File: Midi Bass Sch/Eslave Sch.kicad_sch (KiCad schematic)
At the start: 12 parts, among them J3 E SLAVE ISCP, SW3 E-slave Reset, U2 PIC16F1789

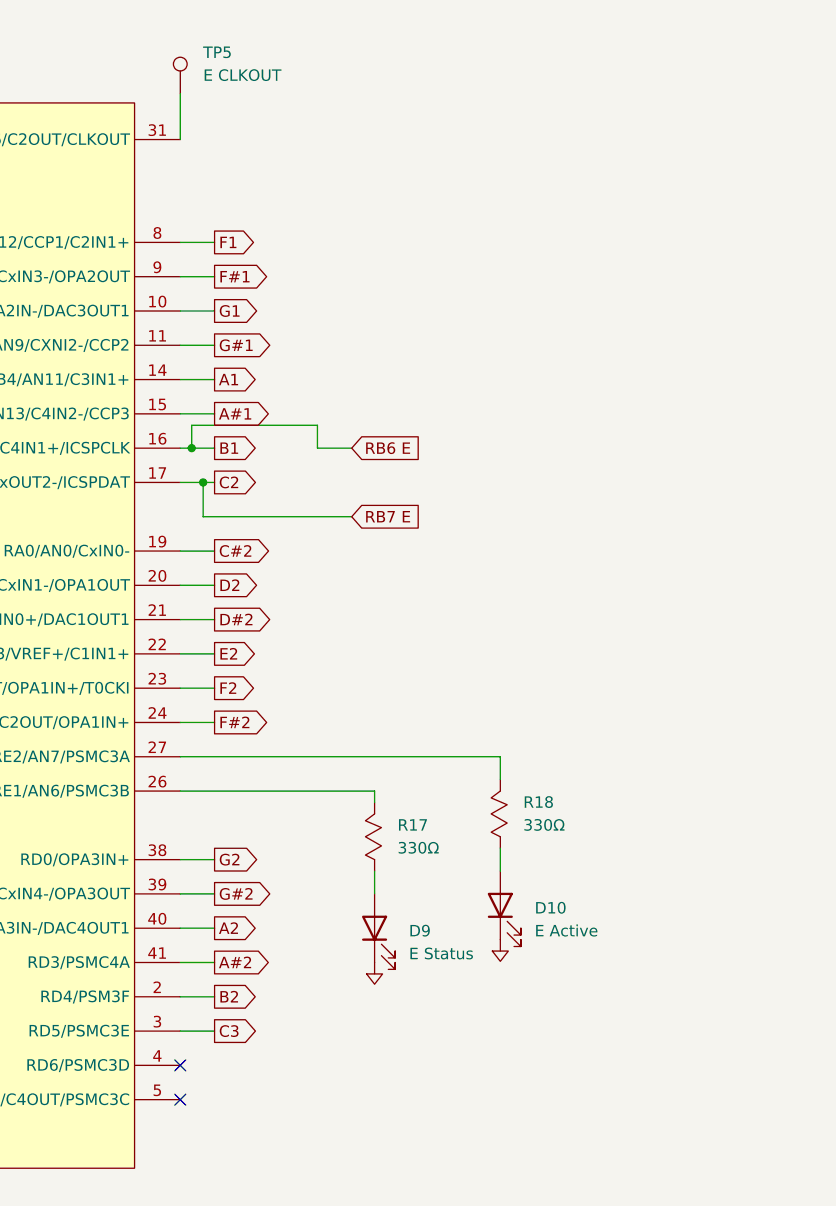
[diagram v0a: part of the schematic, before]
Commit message: finished troubleshooting section
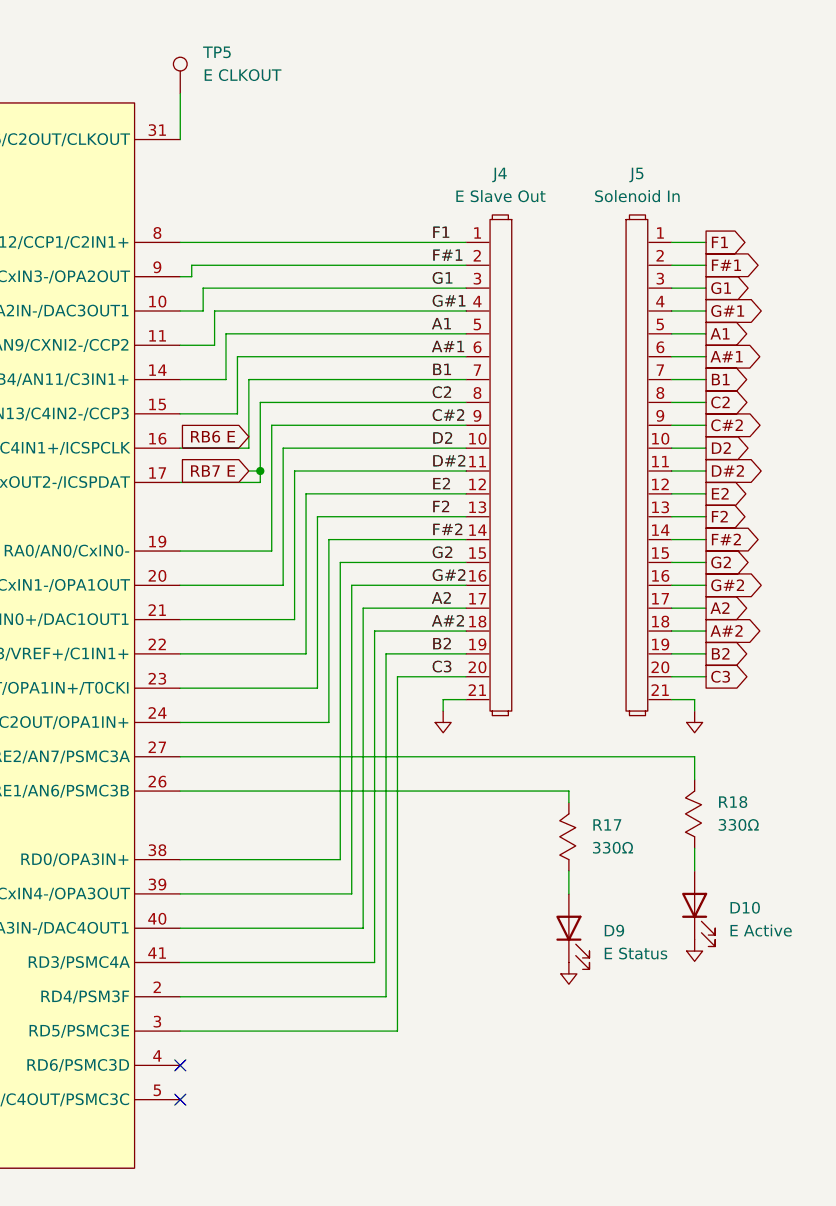
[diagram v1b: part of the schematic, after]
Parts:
- added J4: E Slave Out, symbol Owen's Symbols:Header_1x21
- added J5: Solenoid In, symbol Owen's Symbols:Header_1x21
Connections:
- net A#1: now also J4.6, J5.6
- net A#2: now also J4.18, J5.18
- net A1: now also J4.5, J5.5
- net A2: now also J4.17, J5.17
- net B1: now also J4.7, J5.7
- net B2: now also J4.19, J5.19
- net C#2: now also J4.9, J5.9
- net C2: now also J4.8, J5.8
- net C3: now also J4.20, J5.20
- net D#2: now also J4.11, J5.11
- net D2: now also J4.10, J5.10
- net E2: now also J4.12, J5.12
- net F#1: now also J4.2, J5.2
- net F#2: now also J4.14, J5.14
- net F1: now also J4.1, J5.1
- net F2: now also J4.13, J5.13
- net G#1: now also J4.4, J5.4
- net G#2: now also J4.16, J5.16
- net G1: now also J4.3, J5.3
- net G2: now also J4.15, J5.15
- net GND: now also J4.21, J5.21
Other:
- moved on the sheet: D10, D9, R17, R18
